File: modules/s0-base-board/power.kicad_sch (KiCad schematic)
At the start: 34 parts, among them J2 Screw_Terminal_01x02, J3 BAT_JST_01x02, Q1 PMOS, Q2 2N5401, Q3 IRF4905STRLPBF, U1 MCP73831-2-OT, U2 XL1509-5.0, U3 LM2575S-3.3(UMW)

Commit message: chore: finalize production files for s0
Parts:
- F1: JLCPCB C3105 -> C3105
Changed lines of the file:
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@@
 			)
 		)
-		(property "JLCPCB" "C3105 "
+		(property "JLCPCB" "C3105"
 			(at 200.66 120.65 90)
 			(effects

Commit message: Prod changes
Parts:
- Q2: JLCPCB (none) -> C147293
- Q3: JLCPCB C2620 -> C2620
- R19, R2: JLCPCB C25531 -> C25744
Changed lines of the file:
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@@
 			)
 		)
-		(property "JLCPCB" " C2620"
+		(property "JLCPCB" "C2620"
 			(at 78.74 53.34 90)
 			(effects
@@
 			)
 		)
-		(property "JLCPCB" "C25531 "
+		(property "JLCPCB" "C25744"
 			(at 43.18 59.69 0)
 			(effects
@@
 			)
 		)
-		(property "JLCPCB" "C25531 "
+		(property "JLCPCB" "C25744"
 			(at 179.07 142.24 0)
 			(effects
@@
 			(effects
 				(font
+					(size 1.27 1.27)
+				)
+				(hide yes)
+			)
+		)
+		(property "JLCPCB" "C147293"
+			(at 62.23 62.23 0)
+			(effects
+				(font

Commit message: fix: populate correct bom
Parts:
- C4: JLCPCB C29199 -> C15850
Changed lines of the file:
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@@
 			)
 		)
-		(property "JLCPCB" "C29199"
+		(property "JLCPCB" "C15850"
 			(at 182.88 62.23 0)
 			(effects

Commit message: fix: add male jumper connections for UART
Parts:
- TP4: now left out of the parts list
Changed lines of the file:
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@@
 		(unit 1)
 		(exclude_from_sim no)
-		(in_bom yes)
+		(in_bom no)
 		(on_board yes)
 		(dnp no)

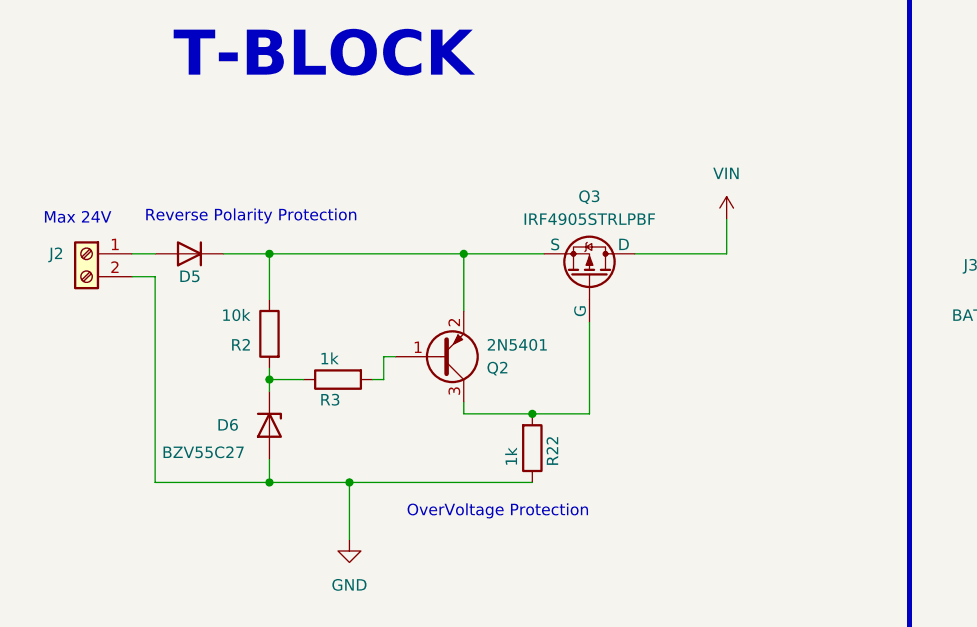
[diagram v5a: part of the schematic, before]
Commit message: feat(production): export gerber and bom for s0 and baseboard
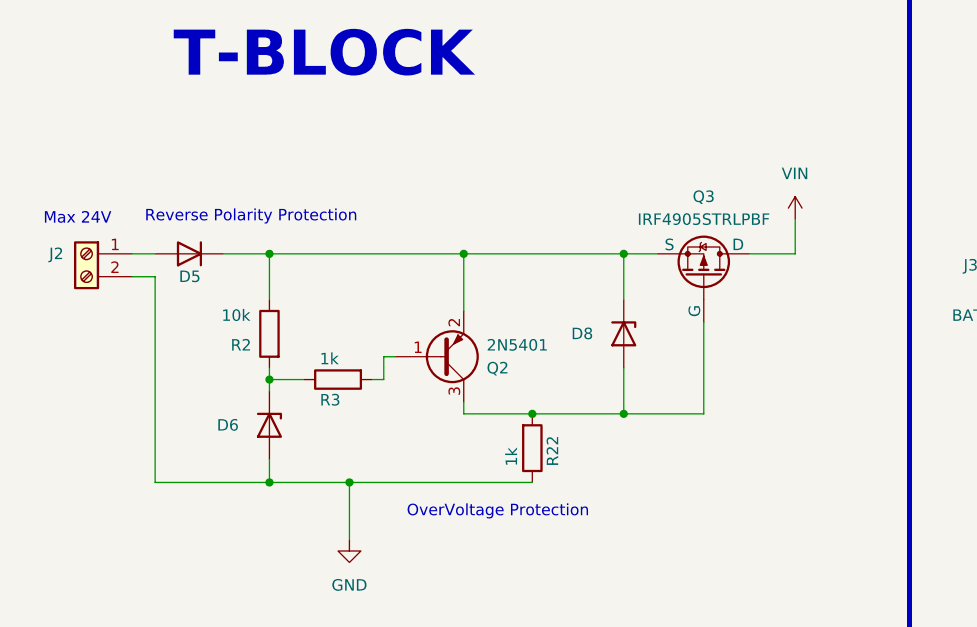
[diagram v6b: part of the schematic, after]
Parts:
- added D8: BZV55C27, Diode_SMD:D_SMA, symbol Diode:BZV55C27
- D6: footprint Diode_SMD:D_MiniMELF -> Diode_SMD:D_SMA; JLCPCB C545374 -> C688905
- Q3: footprint Module:TRANS_IRF3205S -> Package_TO_SOT_SMD:TO-252-2; JLCPCB C2620 -> C397952
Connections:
- net at Q2.3 (C), Q3.2 (G), R22.2: now also D8.2 (A)
- net at D5.1 (K), Q2.2 (E), Q3.3 (S)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: now also D8.1 (K)
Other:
- moved on the sheet: Q3
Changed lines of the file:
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@@
 	)
 	(junction
+		(at 82.55 68.58)
+		(diameter 0)
+		(color 0 0 0 0)
+	)
+	(junction
 		(at 43.18 50.8)
 		(diameter 0)
@@
 	)
 	(junction
+		(at 82.55 50.8)
+		(diameter 0)
+		(color 0 0 0 0)
+	)
+	(junction
 		(at 208.28 120.65)
 		(diameter 0)
@@
 	(wire
 		(pts
-			(xy 83.82 50.8) (xy 93.98 50.8)
+			(xy 96.52 50.8) (xy 101.6 50.8)
 		)
 		(stroke
@@
 	(wire
 		(pts
+			(xy 82.55 68.58) (xy 91.44 68.58)
+		)
+		(stroke
+			(width 0)
+			(type default)
+		)
+	)
+	(wire
+		(pts
 			(xy 267.97 133.35) (xy 267.97 137.16)
 		)
@@
 	(wire
 		(pts
+			(xy 82.55 50.8) (xy 82.55 55.88)
+		)
+		(stroke
+			(width 0)
+			(type default)
+		)
+	)
+	(wire
+		(pts
 			(xy 262.89 49.53) (xy 256.54 49.53)
 		)
@@
 	(wire
 		(pts
-			(xy 64.77 50.8) (xy 73.66 50.8)
+			(xy 64.77 50.8) (xy 82.55 50.8)
 		)
 		(stroke
@@
 	(wire
 		(pts
-			(xy 93.98 50.8) (xy 93.98 46.99)
+			(xy 101.6 50.8) (xy 101.6 46.99)
 		)
 		(stroke
@@
 	(wire
 		(pts
+			(xy 82.55 63.5) (xy 82.55 68.58)
+		)
+		(stroke
+			(width 0)
+			(type default)
+		)
+	)
+	(wire
+		(pts
 			(xy 129.54 52.07) (xy 139.7 52.07)
 		)
@@
 	(wire
 		(pts
+			(xy 82.55 50.8) (xy 86.36 50.8)
+		)
+		(stroke
+			(width 0)
+			(type default)
+		)
+	)
+	(wire
+		(pts
 			(xy 38.1 147.32) (xy 38.1 143.51)
 		)
@@
 	(wire
 		(pts
-			(xy 72.39 68.58) (xy 78.74 68.58)
+			(xy 72.39 68.58) (xy 82.55 68.58)
 		)
 		(stroke
@@
 	(wire
 		(pts
-			(xy 78.74 58.42) (xy 78.74 68.58)
+			(xy 91.44 58.42) (xy 91.44 68.58)
 		)
 		(stroke
@@
 				)
 				(justify left)
+				(hide yes)
 			)
 		)
-		(property "Footprint" "Diode_SMD:D_MiniMELF"
+		(property "Footprint" "Diode_SMD:D_SMA"
 			(at 38.735 69.85 0)
 			(effects
@@
 			)
 		)
-		(property "JLCPCB" "C545374"
+		(property "JLCPCB" "C688905"
 			(at 43.18 69.85 90)
 			(effects
@@
 	(symbol
 		(lib_id "Simulation_SPICE:PMOS")
-		(at 78.74 53.34 270)
+		(at 91.44 53.34 270)
 		(mirror x)
 		(unit 1)
@@
 		(dnp no)
 		(property "Reference" "Q3"
-			(at 78.74 44.45 90)
+			(at 91.44 44.45 90)
 			(effects
 				(font
@@
 		)
 		(property "Value" "IRF4905STRLPBF"
-			(at 78.74 46.99 90)
+			(at 91.44 46.99 90)
 			(effects
 				(font
@@
 			)
 		)
-		(property "Footprint" "Module:TRANS_IRF3205S"
-			(at 81.28 48.26 0)
+		(property "Footprint" "Package_TO_SOT_SMD:TO-252-2"
+			(at 93.98 48.26 0)
 			(effects
 				(font
@@
 		)
 		(property "Datasheet" "https://ngspice.sourceforge.io/docs/ngspice-html-manual/manual.xhtml#cha_MOSFETs"
-			(at 66.04 53.34 0)
+			(at 78.74 53.34 0)
 			(effects
 				(font
@@
 		)
 		(property "Description" "P-MOSFET transistor, drain/source/gate"
-			(at 78.74 53.34 0)
+			(at 91.44 53.34 0)
 			(effects
 				(font
@@
 		)
 		(property "Sim.Device" "PMOS"
-			(at 61.595 53.34 0)
+			(at 74.295 53.34 0)
 			(effects
 				(font
@@
 		)
 		(property "Sim.Type" "VDMOS"
-			(at 59.69 53.34 0)
+			(at 72.39 53.34 0)
 			(effects
 				(font
@@
 		)
 		(property "Sim.Pins" "1=D 2=G 3=S"
-			(at 63.5 53.34 0)
+			(at 76.2 53.34 0)
 			(effects
 				(font
@@
 			)
 		)
-		(property "JLCPCB" "C2620"
-			(at 78.74 53.34 90)
+		(property "JLCPCB" "C397952"
+			(at 91.44 53.34 90)
 			(effects
 				(font
@@
 		)
 		(property "LCSC Part" ""
-			(at 78.74 53.34 0)
+			(at 91.44 53.34 0)
 			(effects
 				(font
@@
 	(symbol
 		(lib_id "power:VCC")
-		(at 93.98 46.99 0)
+		(at 101.6 46.99 0)
 		(unit 1)
 		(exclude_from_sim no)
@@
 		(fields_autoplaced yes)
 		(property "Reference" "#PWR061"
-			(at 93.98 50.8 0)
+			(at 101.6 50.8 0)
 			(effects
 				(font
@@
 		)
 		(property "Value" "VIN"
-			(at 93.98 41.91 0)
+			(at 101.6 41.91 0)
 			(effects
 				(font
@@
 		)
 		(property "Footprint" ""
-			(at 93.98 46.99 0)
+			(at 101.6 46.99 0)
 			(effects
 				(font
@@
 		)
 		(property "Datasheet" ""
-			(at 93.98 46.99 0)
+			(at 101.6 46.99 0)
 			(effects
 				(font
@@
 		)
 		(property "Description" "Power symbol creates a global label with name \"VCC\""
-			(at 93.98 46.99 0)
+			(at 101.6 46.99 0)
 			(effects
 				(font
@@
 					(unit 1)
 				)
+			)
+		)
+	)
+	(symbol
+		(lib_id "Diode:BZV55C27")
+		(at 82.55 59.69 270)
+		(unit 1)
+		(exclude_from_sim no)
+		(in_bom yes)
+		(on_board yes)
+		(dnp no)
+		(property "Reference" "D8"
+			(at 76.708 59.69 90)
+			(effects
+				(font
+					(size 1.27 1.27)
+				)
+				(justify left)
+			)
+		)
+		(property "Value" "BZV55C27"
+			(at 70.612 62.738 90)
+			(effects
+				(font
+					(size 1.27 1.27)
+				)
+				(justify left)
+				(hide yes)
+			)
+		)
+		(property "Footprint" "Diode_SMD:D_SMA"
+			(at 78.105 59.69 0)
+			(effects
+				(font
+					(size 1.27 1.27)
+				)
+				(hide yes)
+			)
+		)
+		(property "Datasheet" "https://assets.nexperia.com/documents/data-sheet/BZV55_SER.pdf"
+			(at 82.55 59.69 0)
+			(effects
+				(font
+					(size 1.27 1.27)
+				)
+				(hide yes)
+			)
+		)
+		(property "Description" "27V, 500mW, 5%, Zener diode, MiniMELF"
+			(at 82.55 59.69 0)
+			(effects
+				(font
+					(size 1.27 1.27)
+				)
+				(hide yes)
+			)
+		)
+		(property "JLCPCB" "C151791"
+			(at 82.55 59.69 90)
+			(effects
+				(font
+					(size 1.27 1.27)
+				)
+				(hide yes)
+			)
+		)
+		(property "LCSC Part" ""
+			(at 82.55 59.69 0)
+			(effects
+				(font
+					(size 1.27 1.27)
+				)
+				(hide yes)
+			)
+		)
+		(pin "1"
+		)
+		(pin "2"
+		)
+		(instances
+			(project "s0-base-board"
+				(path "/30a07aa9-a4c6-42ad-8aa6-f5766a70e64f/c8f0bed1-a3c6-4de4-ad0b-f2169564ca41"
+					(reference "D8")
+					(unit 1)
+				)
